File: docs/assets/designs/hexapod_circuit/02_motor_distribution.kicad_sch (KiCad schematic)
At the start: 4 parts, among them J2 XT30 to actuator, J3 XT30 to actuator

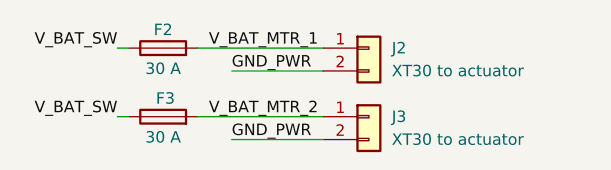
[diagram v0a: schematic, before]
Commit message: Add files via upload
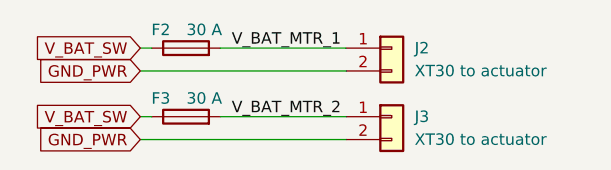
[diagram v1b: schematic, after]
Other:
- moved on the sheet: F2, F3, J2, J3
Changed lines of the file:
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@@
 	(wire
 		(pts
-			(xy 31.75 24.13) (xy 45.72 24.13)
-		)
-		(stroke
-			(width 0)
-			(type default)
-		)
-	)
-	(wire
-		(pts
-			(xy 22.86 16.51) (xy 24.13 16.51)
-		)
-		(stroke
-			(width 0)
-			(type default)
-		)
-	)
-	(wire
-		(pts
-			(xy 31.75 16.51) (xy 45.72 16.51)
-		)
-		(stroke
-			(width 0)
-			(type default)
-		)
-	)
-	(wire
-		(pts
-			(xy 22.86 24.13) (xy 24.13 24.13)
-		)
-		(stroke
-			(width 0)
-			(type default)
-		)
-	)
-	(wire
-		(pts
-			(xy 35.56 19.05) (xy 45.72 19.05)
-		)
-		(stroke
-			(width 0)
-			(type default)
-		)
-	)
-	(wire
-		(pts
-			(xy 35.56 26.67) (xy 45.72 26.67)
+			(xy 34.29 24.13) (xy 48.26 24.13)
+		)
+		(stroke
+			(width 0)
+			(type default)
+		)
+	)
+	(wire
+		(pts
+			(xy 25.4 16.51) (xy 26.67 16.51)
+		)
+		(stroke
+			(width 0)
+			(type default)
+		)
+	)
+	(wire
+		(pts
+			(xy 34.29 16.51) (xy 48.26 16.51)
+		)
+		(stroke
+			(width 0)
+			(type default)
+		)
+	)
+	(wire
+		(pts
+			(xy 25.4 24.13) (xy 26.67 24.13)
+		)
+		(stroke
+			(width 0)
+			(type default)
+		)
+	)
+	(wire
+		(pts
+			(xy 25.4 19.05) (xy 48.26 19.05)
+		)
+		(stroke
+			(width 0)
+			(type default)
+		)
+	)
+	(wire
+		(pts
+			(xy 25.4 26.67) (xy 48.26 26.67)
 		)
 		(stroke
@@
 	)
 	(label "V_BAT_MTR_1"
-		(at 33.02 16.51 0)
+		(at 35.56 16.51 0)
 		(effects
 			(font
@@
 		)
 	)
-	(label "GND_PWR"
-		(at 35.56 19.05 0)
+	(label "V_BAT_MTR_2"
+		(at 35.56 24.13 0)
 		(effects
 			(font
@@
 		)
 	)
-	(label "V_BAT_MTR_2"
-		(at 33.02 24.13 0)
-		(effects
-			(font
-				(size 1.27 1.27)
-			)
-			(justify left bottom)
-		)
-	)
-	(label "V_BAT_SW"
-		(at 22.86 24.13 180)
-		(effects
-			(font
-				(size 1.27 1.27)
-			)
-			(justify right bottom)
-		)
-	)
-	(label "V_BAT_SW"
-		(at 22.86 16.51 180)
-		(effects
-			(font
-				(size 1.27 1.27)
-			)
-			(justify right bottom)
-		)
-	)
-	(label "GND_PWR"
-		(at 35.56 26.67 0)
-		(effects
-			(font
-				(size 1.27 1.27)
-			)
-			(justify left bottom)
+	(global_label "V_BAT_SW"
+		(shape input)
+		(at 25.4 24.13 180)
+		(fields_autoplaced yes)
+		(effects
+			(font
+				(size 1.27 1.27)
+			)
+			(justify right)
+		)
+		(property "Intersheetrefs" "${INTERSHEET_REFS}"
+			(at 13.4039 24.13 0)
+			(effects
+				(font
+					(size 1.27 1.27)
+				)
+				(justify right)
+				(hide yes)
+			)
+		)
+	)
+	(global_label "V_BAT_SW"
+		(shape input)
+		(at 25.4 16.51 180)
+		(fields_autoplaced yes)
+		(effects
+			(font
+				(size 1.27 1.27)
+			)
+			(justify right)
+		)
+		(property "Intersheetrefs" "${INTERSHEET_REFS}"
+			(at 13.4039 16.51 0)
+			(effects
+				(font
+					(size 1.27 1.27)
+				)
+				(justify right)
+				(hide yes)
+			)
+		)
+	)
+	(global_label "GND_PWR"
+		(shape input)
+		(at 25.4 26.67 180)
+		(fields_autoplaced yes)
+		(effects
+			(font
+				(size 1.27 1.27)
+			)
+			(justify right)
+		)
+		(property "Intersheetrefs" "${INTERSHEET_REFS}"
+			(at 13.5853 26.67 0)
+			(effects
+				(font
+					(size 1.27 1.27)
+				)
+				(justify right)
+				(hide yes)
+			)
+		)
+	)
+	(global_label "GND_PWR"
+		(shape input)
+		(at 25.4 19.05 180)
+		(fields_autoplaced yes)
+		(effects
+			(font
+				(size 1.27 1.27)
+			)
+			(justify right)
+		)
+		(property "Intersheetrefs" "${INTERSHEET_REFS}"
+			(at 13.5853 19.05 0)
+			(effects
+				(font
+					(size 1.27 1.27)
+				)
+				(justify right)
+				(hide yes)
+			)
 		)
 	)
 	(symbol
 		(lib_id "Connector_Generic:Conn_01x02")
-		(at 50.8 24.13 0)
+		(at 53.34 24.13 0)
 		(unit 1)
 		(exclude_from_sim no)
@@
 		(fields_autoplaced yes)
 		(property "Reference" "J3"
-			(at 53.34 24.1299 0)
+			(at 55.88 24.1299 0)
 			(effects
 				(font
@@
 		)
 		(property "Value" "XT30 to actuator"
-			(at 53.34 26.6699 0)
+			(at 55.88 26.6699 0)
 			(effects
 				(font
@@
 		)
 		(property "Footprint" ""
-			(at 50.8 24.13 0)
+			(at 53.34 24.13 0)
 			(effects
 				(font
@@
 		)
 		(property "Datasheet" "~"
-			(at 50.8 24.13 0)
+			(at 53.34 24.13 0)
 			(effects
 				(font
@@
 		)
 		(property "Description" "Generic connector, single row, 01x02, script generated (kicad-library-utils/schlib/autogen/connector/)"
-			(at 50.8 24.13 0)
+			(at 53.34 24.13 0)
 			(effects
 				(font
@@
 	(symbol
 		(lib_id "Device:Fuse")
-		(at 27.94 24.13 90)
+		(at 30.48 24.13 90)
 		(unit 1)
 		(exclude_from_sim no)
@@
 		(dnp no)
 		(property "Reference" "F3"
-			(at 28.194 22.098 90)
+			(at 27.686 22.098 90)
 			(effects
 				(font
@@
 		)
 		(property "Value" "30 A"
-			(at 27.94 26.416 90)
+			(at 32.512 22.098 90)
 			(effects
 				(font
@@
 		)
 		(property "Footprint" ""
-			(at 27.94 25.908 90)
+			(at 30.48 25.908 90)
 			(effects
 				(font
@@
 		)
 		(property "Datasheet" "~"
-			(at 27.94 24.13 0)
+			(at 30.48 24.13 0)
 			(effects
 				(font
@@
 		)
 		(property "Description" "Fuse"
-			(at 27.94 24.13 0)
+			(at 30.48 24.13 0)
 			(effects
 				(font
@@
 	(symbol
 		(lib_id "Device:Fuse")
-		(at 27.94 16.51 90)
+		(at 30.48 16.51 90)
 		(unit 1)
 		(exclude_from_sim no)
@@
 		(dnp no)
 		(property "Reference" "F2"
-			(at 27.94 14.478 90)
+			(at 27.686 14.478 90)
 			(effects
 				(font
@@
 		)
 		(property "Value" "30 A"
-			(at 27.94 18.796 90)
+			(at 32.512 14.478 90)
 			(effects
 				(font
@@
 		)
 		(property "Footprint" ""
-			(at 27.94 18.288 90)
+			(at 30.48 18.288 90)
 			(effects
 				(font
@@
 		)
 		(property "Datasheet" "~"
-			(at 27.94 16.51 0)
+			(at 30.48 16.51 0)
 			(effects
 				(font
@@
 		)
 		(property "Description" "Fuse"
-			(at 27.94 16.51 0)
+			(at 30.48 16.51 0)
 			(effects
 				(font
@@
 	(symbol
 		(lib_id "Connector_Generic:Conn_01x02")
-		(at 50.8 16.51 0)
+		(at 53.34 16.51 0)
 		(unit 1)
 		(exclude_from_sim no)
@@
 		(fields_autoplaced yes)
 		(property "Reference" "J2"
-			(at 53.34 16.5099 0)
+			(at 55.88 16.5099 0)
 			(effects
 				(font
@@
 		)
 		(property "Value" "XT30 to actuator"
-			(at 53.34 19.0499 0)
+			(at 55.88 19.0499 0)
 			(effects
 				(font
@@
 		)
 		(property "Footprint" ""
-			(at 50.8 16.51 0)
+			(at 53.34 16.51 0)
 			(effects
 				(font
@@
 		)
 		(property "Datasheet" "~"
-			(at 50.8 16.51 0)
+			(at 53.34 16.51 0)
 			(effects
 				(font
@@
 		)
 		(property "Description" "Generic connector, single row, 01x02, script generated (kicad-library-utils/schlib/autogen/connector/)"
-			(at 50.8 16.51 0)
-			(effects
-				(font
+			(at 53.34 16.51 0)
+			(effects
+				(font

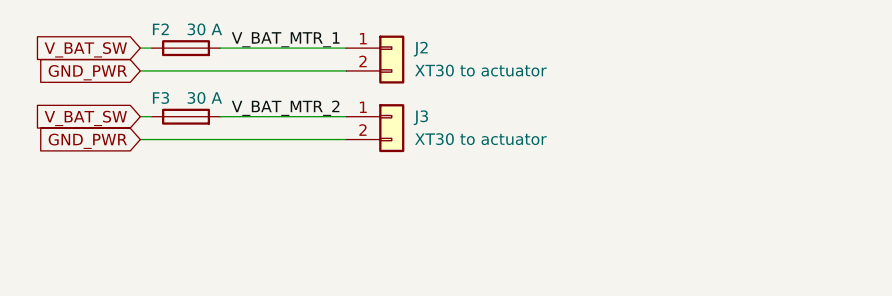
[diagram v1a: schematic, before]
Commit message: upload latest schematic version
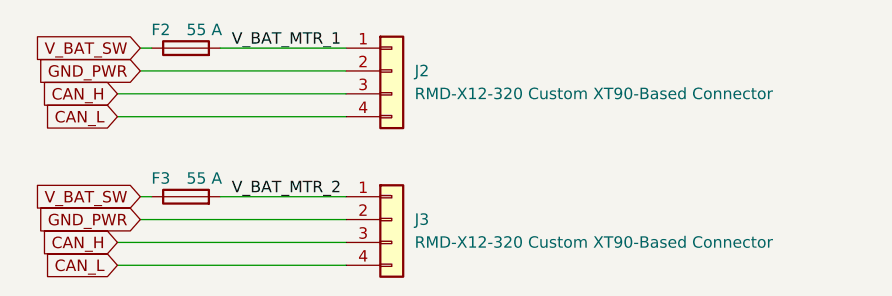
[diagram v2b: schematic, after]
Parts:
- removed J2, J3: XT30 to actuator, symbol Connector_Generic:Conn_01x02
- added J2, J3: RMD-X12-320 Custom XT90-Based Connector, symbol Connector_Generic:Conn_01x04
- F2, F3: value 30 A -> 55 A
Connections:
- net GND_PWR: now also J2.2 (Pin_2), J3.2 (Pin_2)
- net V_BAT_MTR_1: now also J2.1 (Pin_1)
- net V_BAT_MTR_2: now also J3.1 (Pin_1)
- new net CAN_H: J2.3 (Pin_3), J3.3 (Pin_3)
- new net CAN_L: J2.4 (Pin_4), J3.4 (Pin_4)
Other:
- moved on the sheet: F3
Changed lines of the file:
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@@
 	(wire
 		(pts
-			(xy 34.29 24.13) (xy 48.26 24.13)
+			(xy 34.29 33.02) (xy 48.26 33.02)
 		)
 		(stroke
@@
 	(wire
 		(pts
+			(xy 22.86 40.64) (xy 48.26 40.64)
+		)
+		(stroke
+			(width 0)
+			(type default)
+		)
+	)
+	(wire
+		(pts
 			(xy 34.29 16.51) (xy 48.26 16.51)
 		)
@@
 	(wire
 		(pts
-			(xy 25.4 24.13) (xy 26.67 24.13)
+			(xy 25.4 33.02) (xy 26.67 33.02)
+		)
+		(stroke
+			(width 0)
+			(type default)
+		)
+	)
+	(wire
+		(pts
+			(xy 22.86 21.59) (xy 48.26 21.59)
+		)
+		(stroke
+			(width 0)
+			(type default)
+		)
+	)
+	(wire
+		(pts
+			(xy 48.26 24.13) (xy 22.86 24.13)
+		)
+		(stroke
+			(width 0)
+			(type default)
+		)
+	)
+	(wire
+		(pts
+			(xy 22.86 38.1) (xy 48.26 38.1)
 		)
 		(stroke
@@
 	(wire
 		(pts
-			(xy 25.4 26.67) (xy 48.26 26.67)
+			(xy 25.4 35.56) (xy 48.26 35.56)
 		)
 		(stroke
@@
 	)
 	(label "V_BAT_MTR_2"
-		(at 35.56 24.13 0)
+		(at 35.56 33.02 0)
 		(effects
 			(font
@@
 		)
 	)
+	(global_label "CAN_L"
+		(shape input)
+		(at 22.86 24.13 180)
+		(fields_autoplaced yes)
+		(effects
+			(font
+				(size 1.27 1.27)
+			)
+			(justify right)
+		)
+		(property "Intersheetrefs" "${INTERSHEET_REFS}"
+			(at 14.19 24.13 0)
+			(effects
+				(font
+					(size 1.27 1.27)
+				)
+				(justify right)
+				(hide yes)
+			)
+		)
+	)
+	(global_label "CAN_H"
+		(shape input)
+		(at 22.86 38.1 180)
+		(fields_autoplaced yes)
+		(effects
+			(font
+				(size 1.27 1.27)
+			)
+			(justify right)
+		)
+		(property "Intersheetrefs" "${INTERSHEET_REFS}"
+			(at 13.8876 38.1 0)
+			(effects
+				(font
+					(size 1.27 1.27)
+				)
+				(justify right)
+				(hide yes)
+			)
+		)
+	)
 	(global_label "V_BAT_SW"
 		(shape input)
-		(at 25.4 24.13 180)
-		(fields_autoplaced yes)
-		(effects
-			(font
-				(size 1.27 1.27)
-			)
-			(justify right)
-		)
-		(property "Intersheetrefs" "${INTERSHEET_REFS}"
-			(at 13.4039 24.13 0)
+		(at 25.4 33.02 180)
+		(fields_autoplaced yes)
+		(effects
+			(font
+				(size 1.27 1.27)
+			)
+			(justify right)
+		)
+		(property "Intersheetrefs" "${INTERSHEET_REFS}"
+			(at 13.4039 33.02 0)
 			(effects
 				(font
@@
 		)
 	)
+	(global_label "CAN_L"
+		(shape input)
+		(at 22.86 40.64 180)
+		(fields_autoplaced yes)
+		(effects
+			(font
+				(size 1.27 1.27)
+			)
+			(justify right)
+		)
+		(property "Intersheetrefs" "${INTERSHEET_REFS}"
+			(at 14.19 40.64 0)
+			(effects
+				(font
+					(size 1.27 1.27)
+				)
+				(justify right)
+				(hide yes)
+			)
+		)
+	)
 	(global_label "GND_PWR"
 		(shape input)
-		(at 25.4 26.67 180)
-		(fields_autoplaced yes)
-		(effects
-			(font
-				(size 1.27 1.27)
-			)
-			(justify right)
-		)
-		(property "Intersheetrefs" "${INTERSHEET_REFS}"
-			(at 13.5853 26.67 0)
+		(at 25.4 35.56 180)
+		(fields_autoplaced yes)
+		(effects
+			(font
+				(size 1.27 1.27)
+			)
+			(justify right)
+		)
+		(property "Intersheetrefs" "${INTERSHEET_REFS}"
+			(at 13.5853 35.56 0)
 			(effects
 				(font
@@
 		)
 	)
+	(global_label "CAN_H"
+		(shape input)
+		(at 22.86 21.59 180)
+		(fields_autoplaced yes)
+		(effects
+			(font
+				(size 1.27 1.27)
+			)
+			(justify right)
+		)
+		(property "Intersheetrefs" "${INTERSHEET_REFS}"
+			(at 13.8876 21.59 0)
+			(effects
+				(font
+					(size 1.27 1.27)
+				)
+				(justify right)
+				(hide yes)
+			)
+		)
+	)
 	(symbol
-		(lib_id "Connector_Generic:Conn_01x02")
-		(at 53.34 24.13 0)
+		(lib_id "Connector_Generic:Conn_01x04")
+		(at 53.34 19.05 0)
 		(unit 1)
 		(exclude_from_sim no)
@@
 		(dnp no)
 		(fields_autoplaced yes)
-		(property "Reference" "J3"
-			(at 55.88 24.1299 0)
+		(property "Reference" "J2"
+			(at 55.88 19.0499 0)
 			(effects
 				(font
@@
 			)
 		)
-		(property "Value" "XT30 to actuator"
-			(at 55.88 26.6699 0)
+		(property "Value" "RMD-X12-320 Custom XT90-Based Connector"
+			(at 55.88 21.5899 0)
 			(effects
 				(font
@@
 		)
 		(property "Footprint" ""
-			(at 53.34 24.13 0)
+			(at 53.34 19.05 0)
 			(effects
 				(font
@@
 		)
 		(property "Datasheet" "~"
-			(at 53.34 24.13 0)
-			(effects
-				(font
-					(size 1.27 1.27)
-				)
-				(hide yes)
-			)
-		)
-		(property "Description" "Generic connector, single row, 01x02, script generated (kicad-library-utils/schlib/autogen/connector/)"
-			(at 53.34 24.13 0)
-			(effects
-				(font
-					(size 1.27 1.27)
-				)
-				(hide yes)
-			)
+			(at 53.34 19.05 0)
+			(effects
+				(font
+					(size 1.27 1.27)
+				)
+				(hide yes)
+			)
+		)
+		(property "Description" "Generic connector, single row, 01x04, script generated (kicad-library-utils/schlib/autogen/connector/)"
+			(at 53.34 19.05 0)
+			(effects
+				(font
+					(size 1.27 1.27)
+				)
+				(hide yes)
+			)
+		)
+		(pin "3"
+		)
+		(pin "2"
 		)
 		(pin "1"
 		)
-		(pin "2"
+		(pin "4"
 		)
 		(instances
-			(project "hexapod_circuit"
+			(project ""
 				(path "/70bcc270-2cb0-459e-9f52-45e02a660bef/7df8a293-c782-4038-947d-fb3fc39b3078"
-					(reference "J3")
+					(reference "J2")
 					(unit 1)
 				)
@@
 	(symbol
 		(lib_id "Device:Fuse")
-		(at 30.48 24.13 90)
+		(at 30.48 33.02 90)
 		(unit 1)
 		(exclude_from_sim no)
@@
 		(dnp no)
 		(property "Reference" "F3"
-			(at 27.686 22.098 90)
-			(effects
-				(font
-					(size 1.27 1.27)
-				)
-			)
-		)
-		(property "Value" "30 A"
-			(at 32.512 22.098 90)
+			(at 27.686 30.988 90)
+			(effects
+				(font
+					(size 1.27 1.27)
+				)
+			)
+		)
+		(property "Value" "55 A"
+			(at 32.512 30.988 90)
 			(effects
 				(font
@@
 		)
 		(property "Footprint" ""
-			(at 30.48 25.908 90)
+			(at 30.48 34.798 90)
 			(effects
 				(font
@@
 		)
 		(property "Datasheet" "~"
-			(at 30.48 24.13 0)
+			(at 30.48 33.02 0)
 			(effects
 				(font
@@
 		)
 		(property "Description" "Fuse"
-			(at 30.48 24.13 0)
+			(at 30.48 33.02 0)
 			(effects
 				(font
@@
 			)
 		)
-		(property "Value" "30 A"
+		(property "Value" "55 A"
 			(at 32.512 14.478 90)
 			(effects
@@
 	)
 	(symbol
-		(lib_id "Connector_Generic:Conn_01x02")
-		(at 53.34 16.51 0)
+		(lib_id "Connector_Generic:Conn_01x04")
+		(at 53.34 35.56 0)
 		(unit 1)
 		(exclude_from_sim no)
@@
 		(dnp no)
 		(fields_autoplaced yes)
-		(property "Reference" "J2"
-			(at 55.88 16.5099 0)
+		(property "Reference" "J3"
+			(at 55.88 35.5599 0)
 			(effects
 				(font
@@
 			)
 		)
-		(property "Value" "XT30 to actuator"
-			(at 55.88 19.0499 0)
+		(property "Value" "RMD-X12-320 Custom XT90-Based Connector"
+			(at 55.88 38.0999 0)
 			(effects
 				(font
@@
 		)
 		(property "Footprint" ""
-			(at 53.34 16.51 0)
+			(at 53.34 35.56 0)
 			(effects
 				(font
@@
 		)
 		(property "Datasheet" "~"
-			(at 53.34 16.51 0)
-			(effects
-				(font
-					(size 1.27 1.27)
-				)
-				(hide yes)
-			)
-		)
-		(property "Description" "Generic connector, single row, 01x02, script generated (kicad-library-utils/schlib/autogen/connector/)"
-			(at 53.34 16.51 0)
-			(effects
-				(font
-					(size 1.27 1.27)
-				)
-				(hide yes)
-			)
+			(at 53.34 35.56 0)
+			(effects
+				(font
+					(size 1.27 1.27)
+				)
+				(hide yes)
+			)
+		)
+		(property "Description" "Generic connector, single row, 01x04, script generated (kicad-library-utils/schlib/autogen/connector/)"
+			(at 53.34 35.56 0)
+			(effects
+				(font
+					(size 1.27 1.27)
+				)
+				(hide yes)
+			)
+		)
+		(pin "3"
+		)
+		(pin "2"
 		)
 		(pin "1"
 		)
-		(pin "2"
+		(pin "4"
 		)
 		(instances
-			(project ""
+			(project "hexapod_circuit"
 				(path "/70bcc270-2cb0-459e-9f52-45e02a660bef/7df8a293-c782-4038-947d-fb3fc39b3078"
-					(reference "J2")
+					(reference "J3")
 					(unit 1)
 				)
